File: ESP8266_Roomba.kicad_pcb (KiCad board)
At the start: 2 copper layers, 179.1 x 88.2 mm, 59 parts, among them P1 USB_OTG, P2 UG_62864, Q1 BC849, Q2 2N7002, Q3 BC849, Q4 2N7002, Q5 2N7002, SW1 SW_PUSH, SW2 SW_PUSH, SW3 SW_PUSH, U1 TPS62177, U2 CP2102, U3 74LVC3G14, U4 ESP-12E, X1 MINI_DIN_7

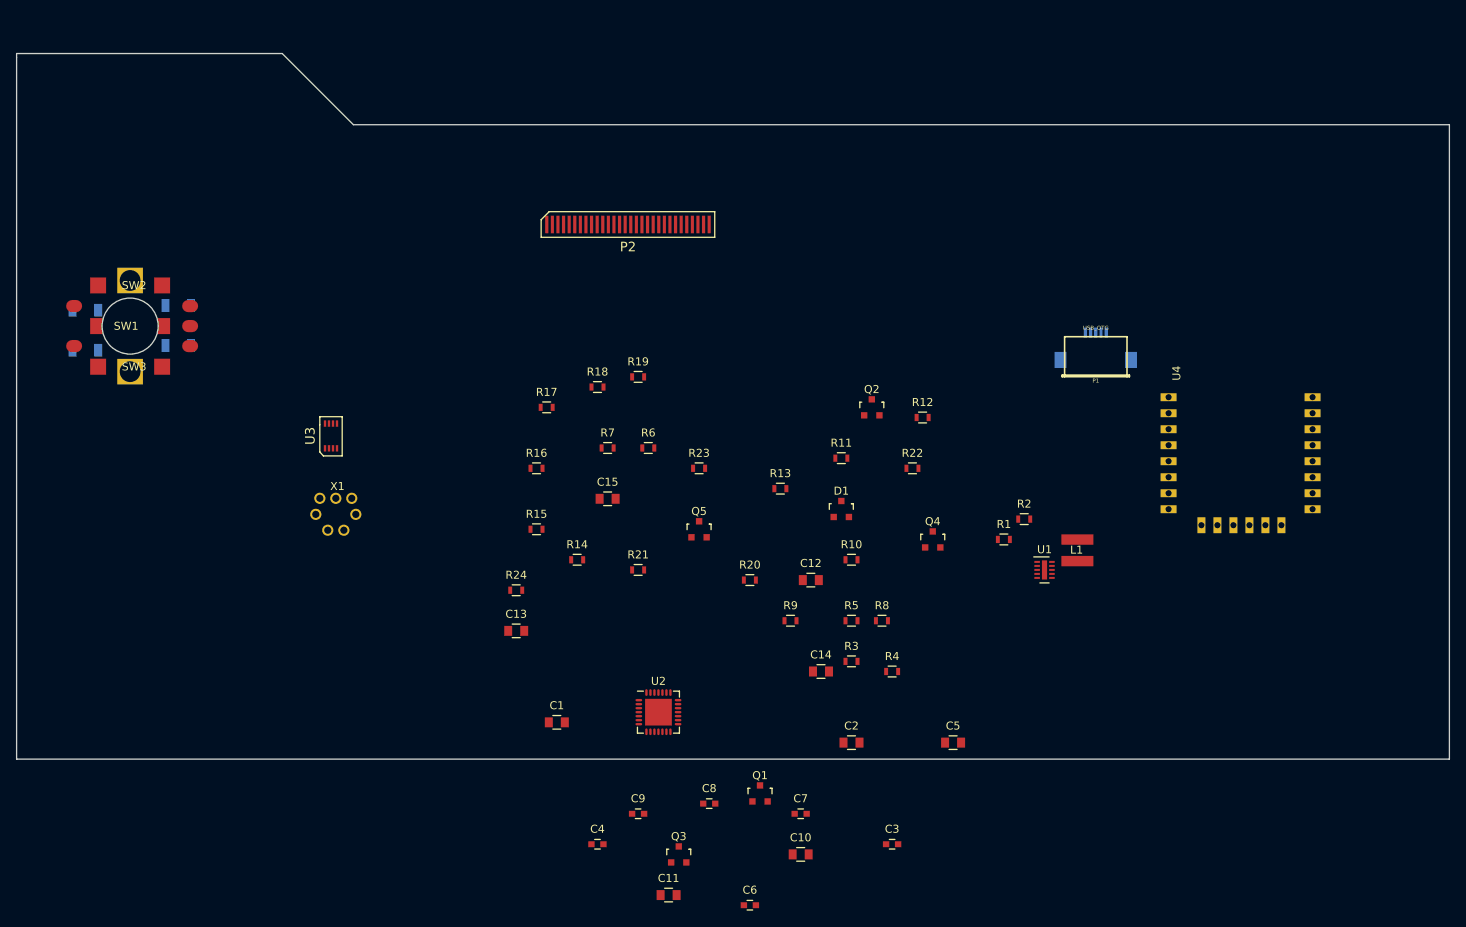
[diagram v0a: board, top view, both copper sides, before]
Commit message: some layout done
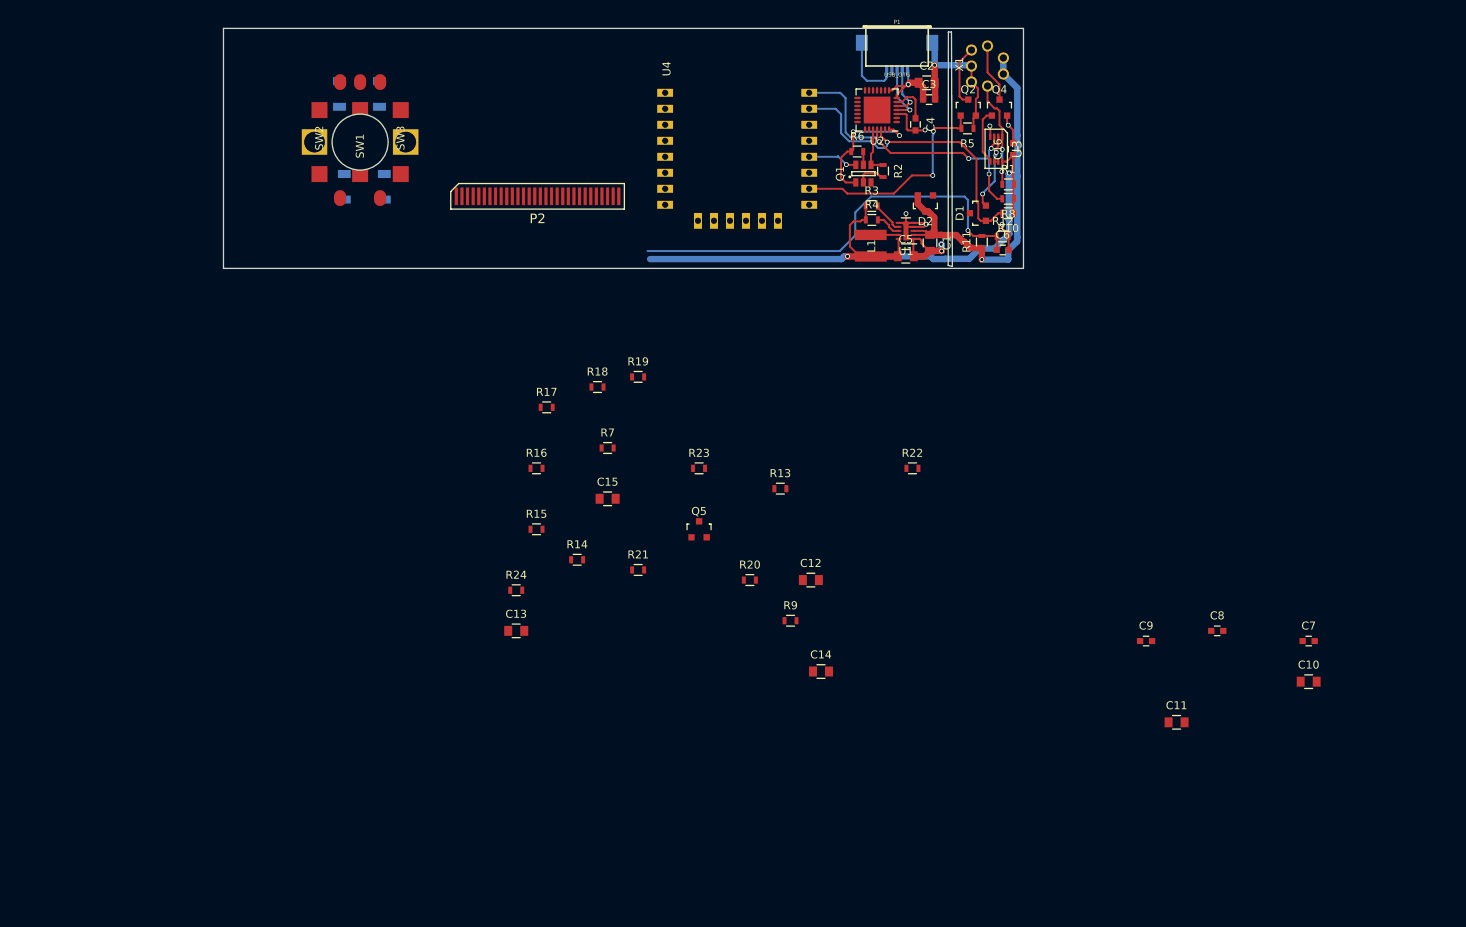
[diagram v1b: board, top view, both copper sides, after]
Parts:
- removed Q3: BC849, TO_SOT_Packages_SMD:SOT-23
- added C16: 100n, Capacitors_SMD:C_0603, F.Cu at (144.7, 55.4)
- added D2: D_Schottky_x2_ACom_AKK, TO_SOT_Packages_SMD:SOT-23, F.Cu at (133.7, 62.1)
- Q1: value BC849 -> DMC204010R; footprint TO_SOT_Packages_SMD:SOT-23 -> TO_SOT_Packages_SMD:SOT-23-6
- moved C4 98.4 mm to (132.5, 52.3), turned to 270 degrees
- moved X1 98.3 mm to (141.1, 45.0), turned to 90 degrees
- moved C3 93.2 mm to (134.2, 49.2)
- moved U3 90.6 mm to (142.6, 55.4), turned to 180 degrees
- moved C6 87.8 mm to (143.4, 68.0)
- moved C2 83.0 mm to (133.9, 47.1)
- moved U2 80.1 mm to (127.7, 50.5), turned to 180 degrees
- moved Q1 78.5 mm to (126.0, 58.4), turned to 90 degrees
- moved C1 75.9 mm to (134.3, 67.1), turned to 270 degrees
- moved U4 73.5 mm to (102.2, 48.3)
- moved C10 67.1 mm to (181.6, 121.9)
- moved C11 67.1 mm to (165.1, 127.0)
- moved C7 67.1 mm to (181.6, 116.8)
- moved C8 67.1 mm to (170.2, 115.6)
- moved C9 67.1 mm to (161.3, 116.8)
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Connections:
- Q1 pad 1: Net-(Q1-Pad1) -> /DTR
- Q1 pad 2: /DTR -> Net-(Q1-Pad2)
- Q1 pad 3: /Switch -> /RST
- R2 pad 2: Net-(Q1-Pad1) -> Net-(Q1-Pad2)
- R6 pad 2: Net-(Q3-Pad1) -> Net-(Q1-Pad5)
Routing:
- net +3V3: track 0.00 -> 81.5 mm, vias 0 -> 2
- net GND: track 0.00 -> 62.5 mm, vias 0 -> 9
- net /ADC: track 0.00 -> 54.1 mm, vias 0 -> 1
- net +12V: track 0.00 -> 48.9 mm, vias 0 -> 1
- net /TXD: track 0.00 -> 39.1 mm, vias 0 -> 4
- net /RXD: track 0.00 -> 38.7 mm, vias 0 -> 1
- net /Roomba_Wake: track 0.00 -> 27.6 mm, vias 0 -> 2
- net /DTR: track 0.00 -> 16.4 mm, vias 0 -> 2
- net Net-(R1-Pad1): track 0.00 -> 13.3 mm, vias 0 -> 2
- net +5V: track 0.00 -> 10.7 mm, vias 0 -> 1
- net Net-(D1-Pad2): track 0.00 -> 9.57 mm, vias 0 -> 2
- net Net-(Q2-Pad3): track 0.00 -> 7.68 mm
- net Net-(P1-Pad3): track 0.00 -> 7.34 mm, vias 0 -> 1
- net Net-(Q4-Pad3): track 0.00 -> 7.32 mm
- net Net-(Q4-Pad1): track 0.00 -> 7.00 mm
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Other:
- board size 179.1 x 88.2 mm -> 100 x 30 mm
- net class high current added: clearance 0.2, trace_width 0.8, via_dia 0.6, via_drill 0.4
- net class small added: clearance 0.2, trace_width 0.15, via_dia 0.6, via_drill 0.4
- rule trace_min: 0.2 -> 0.15
